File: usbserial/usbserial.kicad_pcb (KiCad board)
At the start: 4 copper layers, 50.3 x 28.2 mm, 16 parts, among them J101 Conn_01x06, Q401 MMBT3904, Q402 MMBT3904, U401 USBLC6-2SC6, U402 CH340C

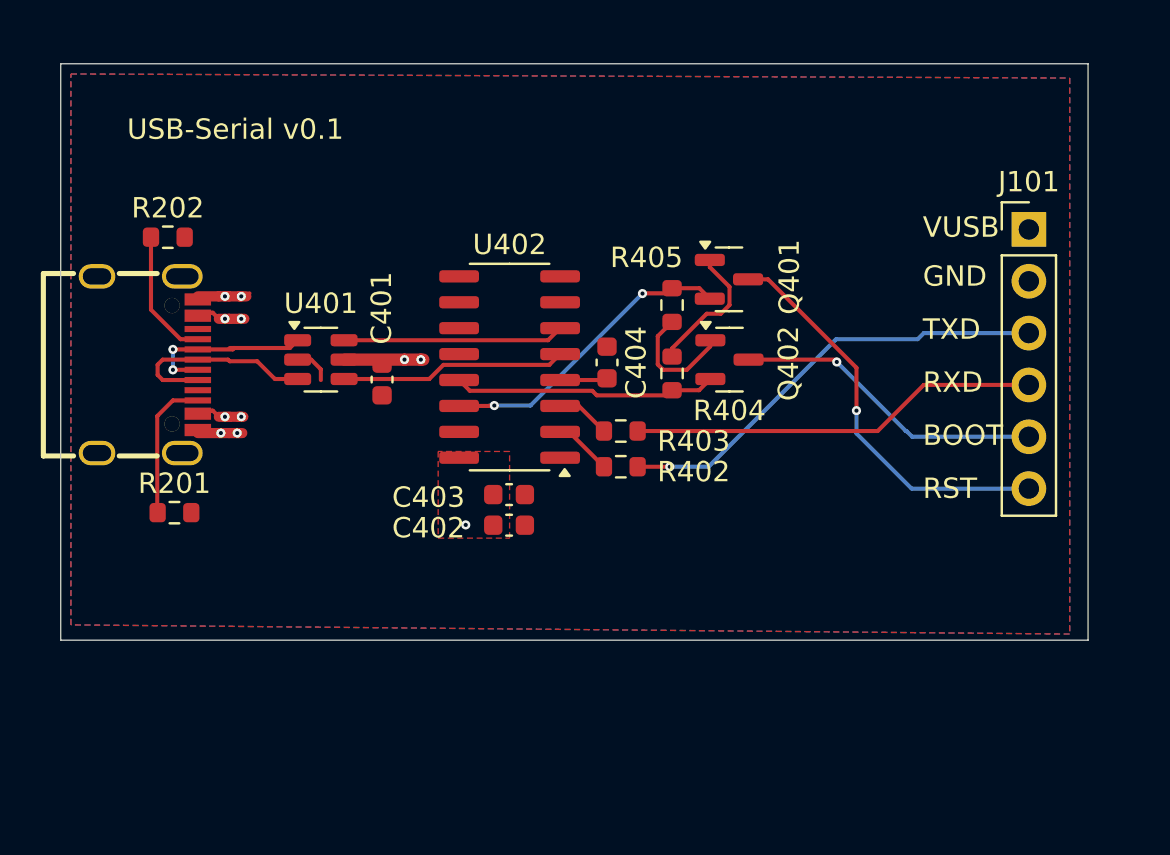
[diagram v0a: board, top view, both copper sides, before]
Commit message: work on usbserial
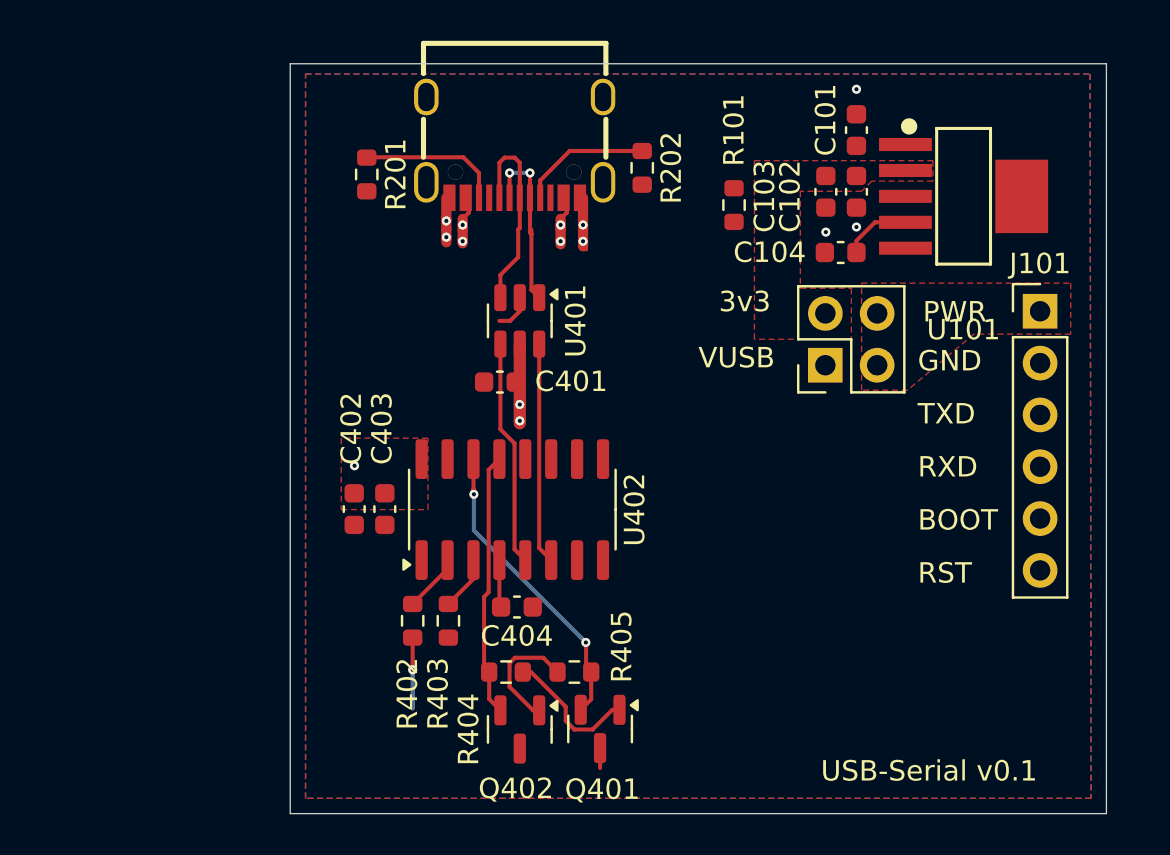
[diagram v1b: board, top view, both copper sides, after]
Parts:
- added C101: 1uF, Capacitor_SMD:C_0603_1608Metric, F.Cu at (52.8, 16.2)
- added C102: 1uF, Capacitor_SMD:C_0603_1608Metric, F.Cu at (52.8, 19.3)
- added C103: 1uF, Capacitor_SMD:C_0603_1608Metric, F.Cu at (51.2, 19.3)
- added C104: 10nF, Capacitor_SMD:C_0603_1608Metric, F.Cu at (52.0, 22.2)
- added J102: Conn_02x02_Counter_Clockwise, Connector_PinHeader_2.54mm:PinHeader_2x02_P2.54mm_Vertical, F.Cu at (51.2, 27.8)
- added R101: 10k, Resistor_SMD:R_0603_1608Metric, F.Cu at (46.8, 19.9)
- added U101: TPS73733DCQ_C5220270, easyeda2kicad:SOT-223-6_L6.5-W3.5-P1.27-LS7.0-BR, F.Cu at (58.0, 19.5)
- moved R202 23.5 mm to (42.2, 18.1), turned to -90 degrees
- moved Q401 22.9 mm to (40.2, 45.6), turned to -90 degrees
- moved USBC201 20.9 mm to (36.0, 17.1), turned to 180 degrees
- moved Q402 20.8 mm to (36.2, 45.6), turned to -90 degrees
- moved R201 19.1 mm to (28.8, 18.4), turned to -90 degrees
- moved R405 18.6 mm to (38.9, 42.8), turned to 0 degrees
- moved R404 16.7 mm to (35.6, 42.8), turned to 180 degrees
- moved C404 12.8 mm to (36.1, 39.6), turned to 180 degrees
- moved R402 12.7 mm to (31.0, 40.3), turned to -90 degrees
- moved R403 12.6 mm to (32.8, 40.3), turned to 90 degrees
- moved U401 9.93 mm to (36.2, 25.6), turned to -90 degrees
- moved C402 7.63 mm to (28.1, 34.8), turned to -90 degrees
- moved U402 6.99 mm to (35.9, 34.9), turned to 90 degrees
- moved C403 6.13 mm to (29.6, 34.8), turned to -90 degrees
- moved C401 5.78 mm to (35.3, 28.6), turned to 180 degrees
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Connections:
- J101 pad 1: /usb_serial/VUSB -> /PWR
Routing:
- net /usb_serial/RXD: track 20.1 -> 0.00 mm
- net /usb_serial/RST: track 19.9 -> 0.98 mm, vias 1 -> 0
- net /usb_serial/TXD: track 22.1 -> 3.73 mm
- net /usb_serial/BOOT: track 15.4 -> 0.00 mm, vias 1 -> 0
- net Net-(U101-NR/FB): track 0.00 -> 3.35 mm
- net GND: vias 4 -> 7
- added copper zone on F.Cu, net /3v3
- added copper zone on F.Cu, net /PWR
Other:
- board size 50.3 x 28.2 mm -> 40 x 36.8 mm
- board text added: "3v3"
- board text added: "PWR"
